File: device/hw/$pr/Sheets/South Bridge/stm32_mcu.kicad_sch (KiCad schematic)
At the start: 36 parts, among them Q2 NPN, Q3 NPN, SW2 SW_SPDT, SW3 SW_Push, U7 STM32F411CEU6, Y1 12.5pF, Y2 18pF

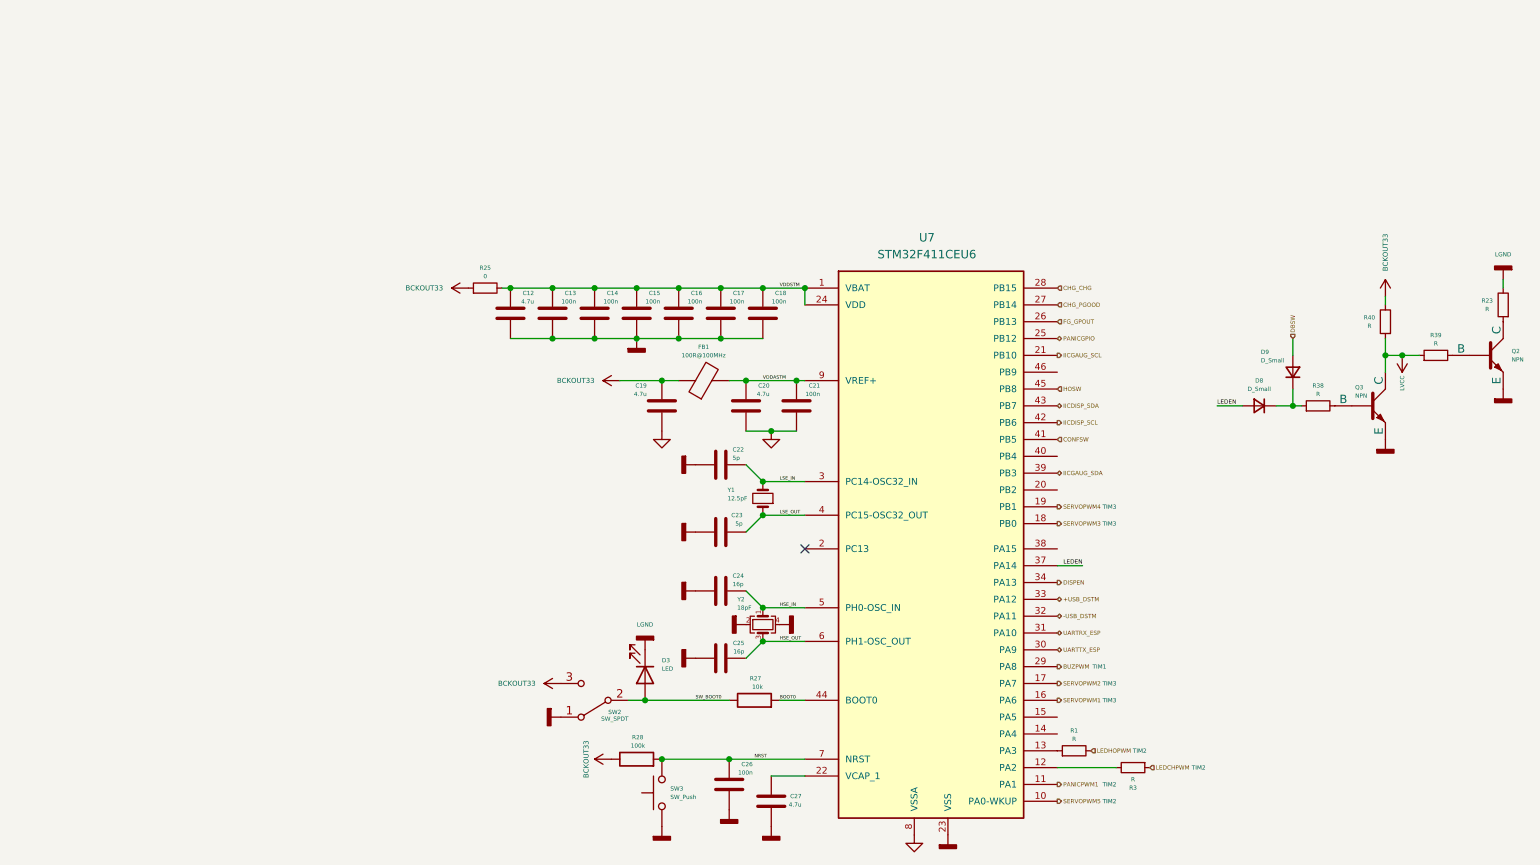
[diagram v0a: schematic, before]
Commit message: application
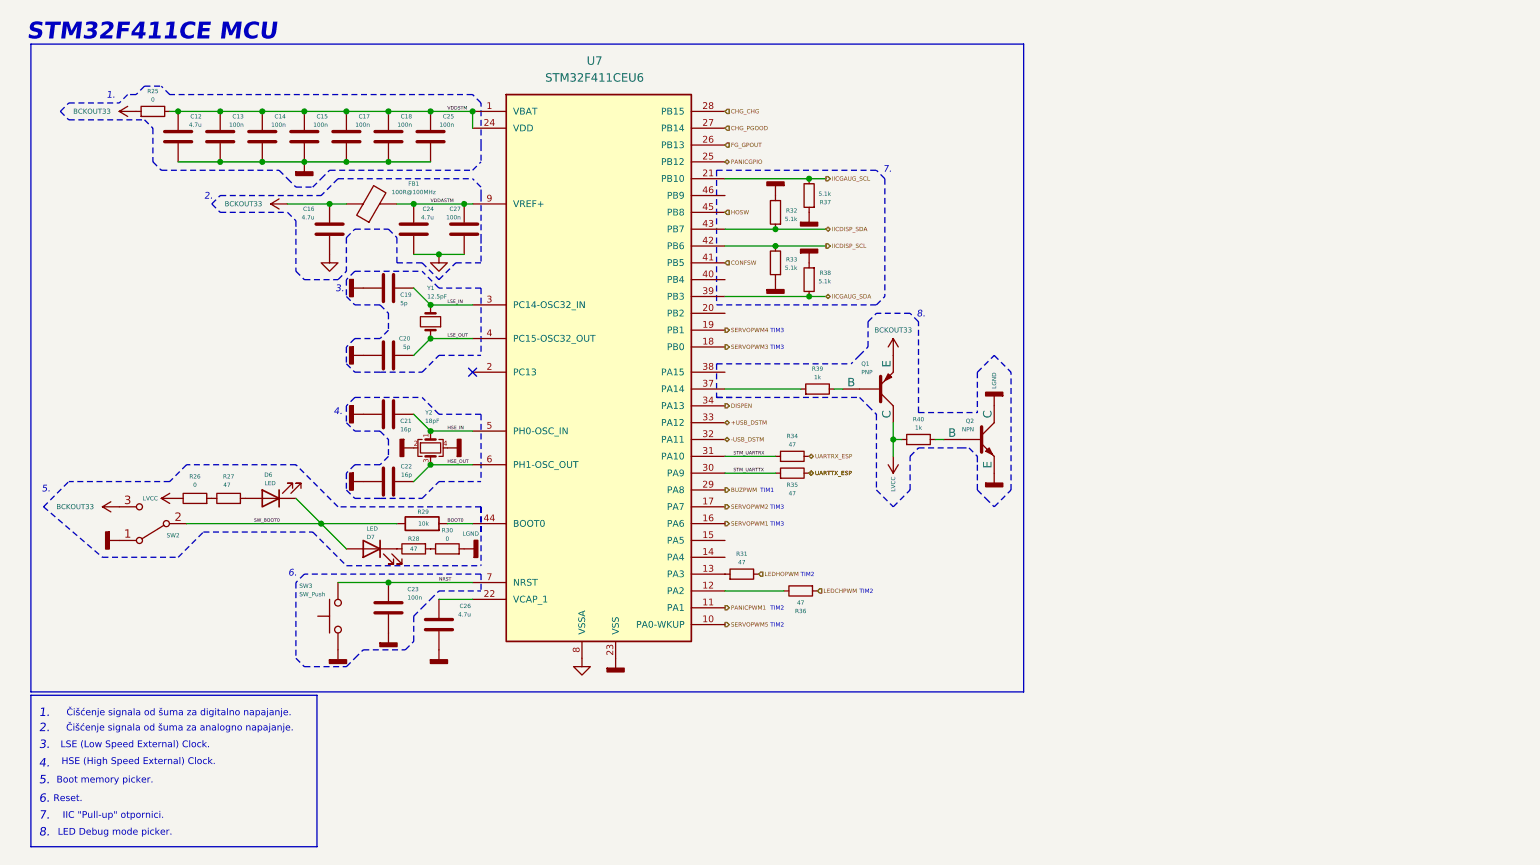
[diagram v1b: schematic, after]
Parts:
- removed D3: LED, LED_SMD:LED_0603_1608Metric, symbol Device:LED
- removed D8, D9: D_Small, Diode_SMD:D_SOD-323, symbol Device:D_Small
- removed Q3: NPN, Package_TO_SOT_SMD:SOT-23, symbol Simulation_SPICE:NPN
- removed R23: R, symbol Device:R_Small
- removed R28: 100k, Resistor_SMD:R_0603_1608Metric, symbol Device:R
- added D6, D7: LED, LED_SMD:LED_0603_1608Metric, symbol Device:LED
- added Q1: PNP, symbol Simulation_SPICE:PNP
- added R26, R30: 0, symbol Device:R_Small
- added R27, R28, R34, R35: 47, symbol Device:R_Small
- added R32, R33, R37: 5.1k, Resistor_SMD:R_0402_1005Metric, symbol Device:R_Small
- R31: renamed from R1; value R -> 47
- R36: renamed from R3; value R -> 47
- R38: value R -> 5.1k; footprint (none) -> Resistor_SMD:R_0402_1005Metric; LCSCPart (none) -> C25905
- R39, R40: value R -> 1k
- renumbered C19 to C16, C16 to C17, C17 to C18, C22 to C19, C23 to C20, C24 to C21, C25 to C22, C26 to C23, C20 to C24, C18 to C25, C27 to C26, C21 to C27, R27 to R29
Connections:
- net BCKOUT33: now also Q1.3 (E); no longer R40.2
- net GNDD: now also R38.1, R32.2, R33.1, R37.1
- net IICDISP_SCL: now also R33.2
- net IICDISP_SDA: now also R32.1
- net IICGAUG_SCL: now also R37.2
- net IICGAUG_SDA: now also R38.2
- net LGND: now also Q2.1 (C), R30.1
- net LVCC: now also Q1.1 (C), R26.2; no longer R39.1
- net SW_BOOT0: now also D6.1 (K), D7.2 (A)
- net UARTRX_ESP: now also R34.2; no longer U7.31 (PA10)
- net UARTTX_ESP: now also R35.2; no longer U7.30 (PA9)
- net at Q2.2 (B): now also R40.2; no longer R39.2
- net LEDEN: no longer names the net of U7.37 (PA14)
- net LEDEN: now also R39.1
- new net: R26.1, R27.2
- new net: R28.1, R30.2
- new net: Q1.2 (B), R39.2
- new net: D6.2 (A), R27.1
- new net: D7.1 (K), R28.2
- new net STM_UARTRX: R34.1, U7.31 (PA10)
- new net STM_UARTTX: R35.1, U7.30 (PA9)
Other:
- note added: "1."
- note added: "2."
- note added: "3."
- note added: "4."
- note added: "5."
- note added: "6."
- note added: "7."
- note added: "8."
- note added: "Boot memory picker."
- note added: "HSE (High Speed External) Clock."
- note added: "IIC "Pull-up" otpornici."
- note added: "LED Debug mode picker."
- note added: "LSE (Low Speed External) Clock."
- note added: "Reset."
- note added: "STM32F411CE MCU"
- note added: "Čišćenje signala od šuma za analogno napajanje."
- note added: "Čišćenje signala od šuma za digitalno napajanje."
- moved on the sheet: C12, C13, C14, C15, C16, C17, C18, C19, C20, C21, C22, C23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
